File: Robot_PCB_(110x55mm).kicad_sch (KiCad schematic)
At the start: 24 parts, among them J1 HC-SR04, Q1 J3, SW1 Switch, U1 L293, U2 AMS1117-5.0, U5 MFRC522 37.5x25mm

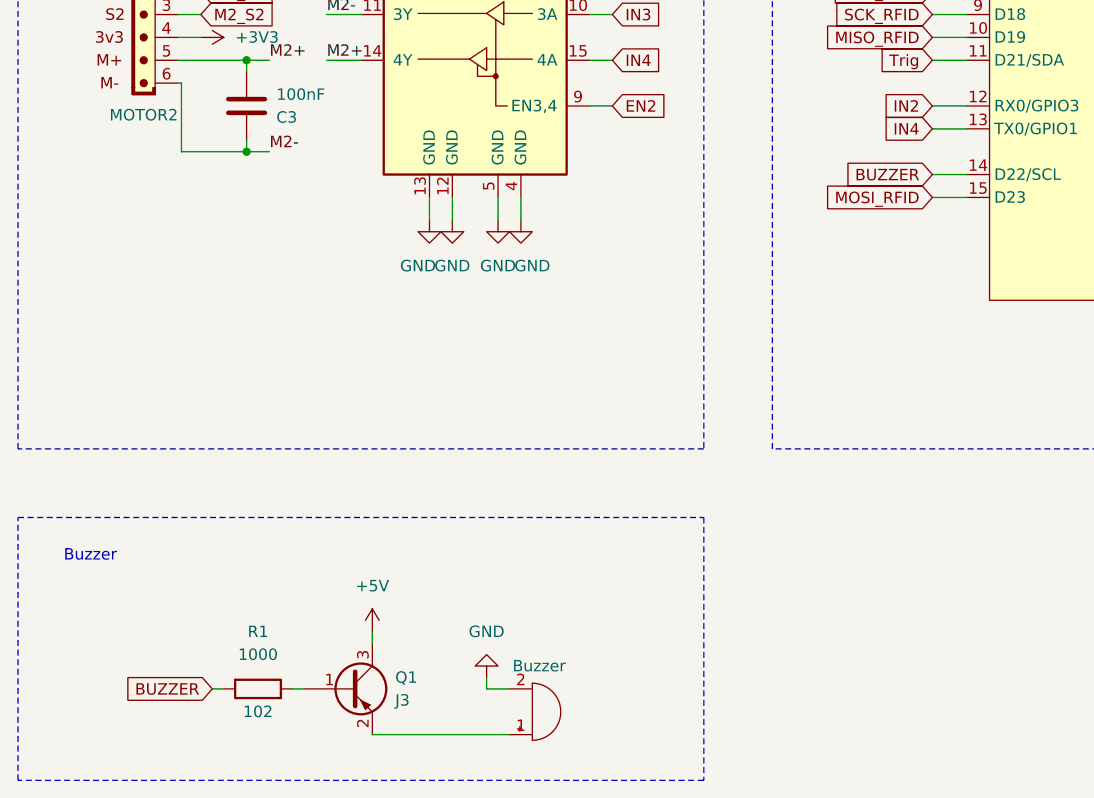
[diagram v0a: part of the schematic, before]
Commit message: Update
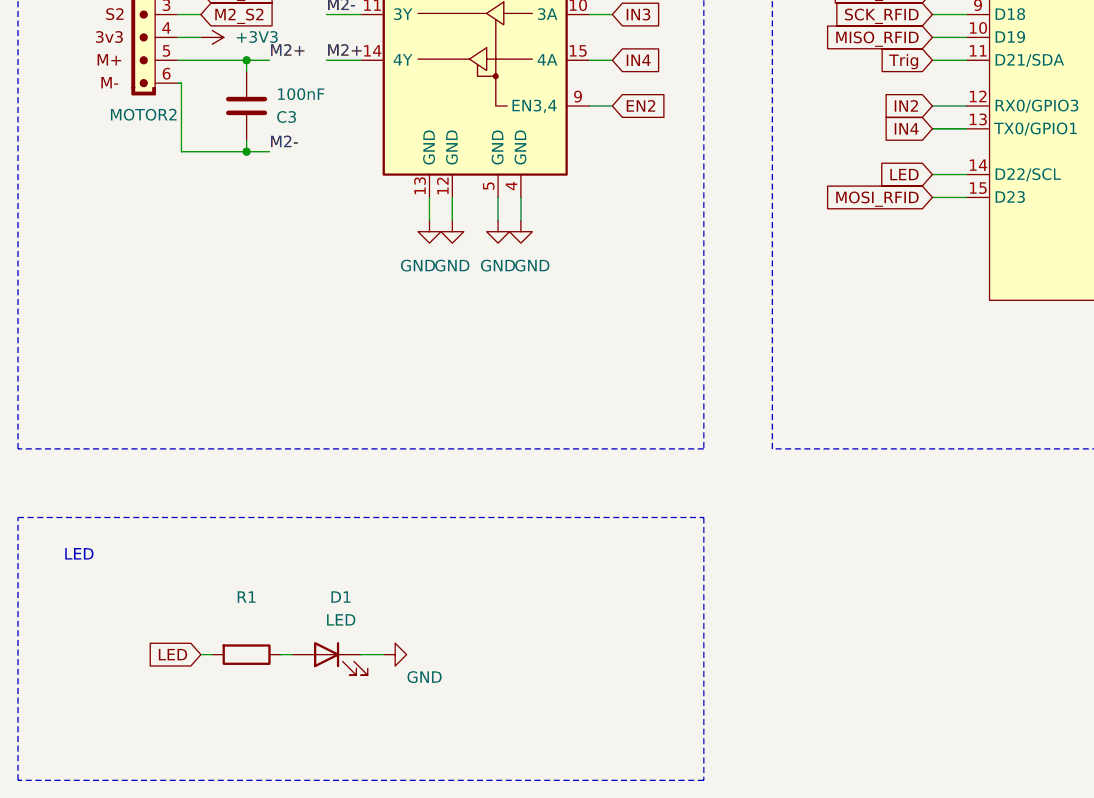
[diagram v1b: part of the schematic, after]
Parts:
- removed BZ1: Buzzer, Buzzer_Beeper:Buzzer_12x9.5RM7.6, symbol Device:Buzzer
- removed Q1: J3, Package_TO_SOT_SMD:SOT-23_Handsoldering, symbol Transistor_BJT:MMBT3906
- added D1: LED, LED_THT:LED_D3.0mm_Clear, symbol Device:LED
- R1: value 1000 -> ~; Campo4 102 -> (none)
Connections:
- net GND: now also D1.1 (K)
- net at R1.1: now also D1.2 (A)
- net BUZZER renamed LED
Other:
- note added: "LED"
- note removed: "Buzzer"
- moved on the sheet: R1
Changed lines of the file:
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@@
-    (stroke (width 0) (type default))
-  )
-  (wire (pts (xy 64.77 172.72) (xy 64.77 173.99))
-    (stroke (width 0) (type default))
-  )
-  (wire (pts (xy 64.77 184.15) (xy 80.01 184.15))
     (stroke (width 0) (type default))
   )
@@
     (stroke (width 0) (type default))
   )
-  (wire (pts (xy 77.47 177.8) (xy 77.47 179.07))
-    (stroke (width 0) (type default))
-  )
   (wire (pts (xy 200.66 44.45) (xy 210.82 44.45))
     (stroke (width 0) (type default))
@@
     (stroke (width 0) (type default))
   )
+  (wire (pts (xy 63.5 175.26) (xy 66.04 175.26))
+    (stroke (width 0) (type default))
+  )
   (wire (pts (xy 127 93.98) (xy 130.81 93.98))
     (stroke (width 0) (type default))
   )
-  (wire (pts (xy 46.99 179.07) (xy 48.26 179.07))
+  (wire (pts (xy 45.72 175.26) (xy 46.99 175.26))
     (stroke (width 0) (type default))
   )
@@
     (stroke (width 0) (type default))
   )
-  (wire (pts (xy 55.88 179.07) (xy 57.15 179.07))
-    (stroke (width 0) (type default))
-  )
   (wire (pts (xy 208.28 33.02) (xy 210.82 33.02))
     (stroke (width 0) (type default))
@@
     (stroke (width 0) (type default))
   )
-  (wire (pts (xy 77.47 179.07) (xy 80.01 179.07))
-    (stroke (width 0) (type default))
-  )
   (wire (pts (xy 91.44 93.98) (xy 88.9 93.98))
     (stroke (width 0) (type default))
@@
   )
   (wire (pts (xy 49.53 93.98) (xy 49.53 92.71))
+    (stroke (width 0) (type default))
+  )
+  (wire (pts (xy 55.88 175.26) (xy 54.61 175.26))
     (stroke (width 0) (type default))
   )
@@
     (effects (font (size 1.27 1.27)) (justify left bottom))
   )
-  (text "Buzzer" (at 30.48 165.1 0)
+  (text "LED" (at 30.48 165.1 0)
     (effects (font (size 1.27 1.27)) (justify left bottom))
   )
@@
     )
   )
-  (global_label "BUZZER" (shape input) (at 46.99 179.07 180) (fields_autoplaced)
-    (effects (font (size 1.27 1.27)) (justify right))
-    (property "Intersheetrefs" "${INTERSHEET_REFS}" (at 36.5663 179.07 0)
-      (effects (font (size 1.27 1.27)) (justify right) hide)
-    )
-  )
-  (global_label "BUZZER" (shape input) (at 127 121.92 180) (fields_autoplaced)
-    (effects (font (size 1.27 1.27)) (justify right))
-    (property "Intersheetrefs" "${INTERSHEET_REFS}" (at 116.5763 121.92 0)
+  (global_label "LED" (shape input) (at 45.72 175.26 180) (fields_autoplaced)
+    (effects (font (size 1.27 1.27)) (justify right))
+    (property "Intersheetrefs" "${INTERSHEET_REFS}" (at 39.2877 175.26 0)
+      (effects (font (size 1.27 1.27)) (justify right) hide)
+    )
+  )
+  (global_label "LED" (shape input) (at 127 121.92 180) (fields_autoplaced)
+    (effects (font (size 1.27 1.27)) (justify right))
+    (property "Intersheetrefs" "${INTERSHEET_REFS}" (at 120.5677 121.92 0)
       (effects (font (size 1.27 1.27)) (justify right) hide)
     )
@@
         (path "/5740c1d8-40a5-48a4-b0ff-1fed8540b5f6"
           (reference "#PWR030") (unit 1)
-        )
-      )
-    )
-  )
-  (symbol (lib_id "power:+5V") (at 64.77 172.72 0) (unit 1)
-    (in_bom yes) (on_board yes) (dnp no) (fields_autoplaced)
-    (property "Reference" "#PWR031" (at 64.77 176.53 0)
-      (effects (font (size 1.27 1.27)) hide)
-    )
-    (property "Value" "+5V" (at 64.77 167.64 0)
-      (effects (font (size 1.27 1.27)))
-    )
-    (property "Footprint" "" (at 64.77 172.72 0)
-      (effects (font (size 1.27 1.27)) hide)
-    )
-    (property "Datasheet" "" (at 64.77 172.72 0)
-      (effects (font (size 1.27 1.27)) hide)
-    )
-    (pin "1")
-    (instances
-      (project "Robot_PCB_(110x55mm)"
-        (path "/5740c1d8-40a5-48a4-b0ff-1fed8540b5f6"
-          (reference "#PWR031") (unit 1)
         )
       )
@@
     )
   )
+  (symbol (lib_id "power:GND") (at 66.04 175.26 90) (unit 1)
+    (in_bom yes) (on_board yes) (dnp no)
+    (property "Reference" "#PWR027" (at 72.39 175.26 0)
+      (effects (font (size 1.27 1.27)) hide)
+    )
+    (property "Value" "GND" (at 68.58 177.8 90)
+      (effects (font (size 1.27 1.27)) (justify right))
+    )
+    (property "Footprint" "" (at 66.04 175.26 0)
+      (effects (font (size 1.27 1.27)) hide)
+    )
+    (property "Datasheet" "" (at 66.04 175.26 0)
+      (effects (font (size 1.27 1.27)) hide)
+    )
+    (pin "1")
+    (instances
+      (project "Robot_PCB_(110x55mm)"
+        (path "/5740c1d8-40a5-48a4-b0ff-1fed8540b5f6"
+          (reference "#PWR027") (unit 1)
+        )
+      )
+    )
+  )
   (symbol (lib_id "Device:R") (at 247.65 34.29 0) (unit 1)
     (in_bom yes) (on_board yes) (dnp no)
@@
     )
   )
-  (symbol (lib_id "Device:R") (at 52.07 179.07 270) (unit 1)
-    (in_bom yes) (on_board yes) (dnp no)
-    (property "Reference" "R1" (at 52.07 172.72 90)
-      (effects (font (size 1.27 1.27)))
-    )
-    (property "Value" "1000" (at 52.07 175.26 90)
-      (effects (font (size 1.27 1.27)))
-    )
-    (property "Footprint" "Resistor_SMD:R_0805_2012Metric_Pad1.20x1.40mm_HandSolder" (at 52.07 177.292 90)
-      (effects (font (size 1.27 1.27)) hide)
-    )
-    (property "Datasheet" "~" (at 52.07 179.07 0)
-      (effects (font (size 1.27 1.27)) hide)
-    )
-    (property "Campo4" "102" (at 52.07 181.61 90)
-      (effects (font (size 1.27 1.27)))
+  (symbol (lib_id "Device:R") (at 50.8 175.26 270) (unit 1)
+    (in_bom yes) (on_board yes) (dnp no)
+    (property "Reference" "R1" (at 50.8 168.91 90)
+      (effects (font (size 1.27 1.27)))
+    )
+    (property "Value" "~" (at 50.8 171.45 90)
+      (effects (font (size 1.27 1.27)))
+    )
+    (property "Footprint" "Resistor_SMD:R_0805_2012Metric_Pad1.20x1.40mm_HandSolder" (at 50.8 173.482 90)
+      (effects (font (size 1.27 1.27)) hide)
+    )
+    (property "Datasheet" "~" (at 50.8 175.26 0)
+      (effects (font (size 1.27 1.27)) hide)
     )
     (pin "1")
@@
         (path "/5740c1d8-40a5-48a4-b0ff-1fed8540b5f6"
           (reference "#PWR04") (unit 1)
-        )
-      )
-    )
-  )
-  (symbol (lib_id "power:GND") (at 77.47 177.8 0) (mirror x) (unit 1)
-    (in_bom yes) (on_board yes) (dnp no)
-    (property "Reference" "#PWR027" (at 77.47 171.45 0)
-      (effects (font (size 1.27 1.27)) hide)
-    )
-    (property "Value" "GND" (at 77.47 172.72 0)
-      (effects (font (size 1.27 1.27)))
-    )
-    (property "Footprint" "" (at 77.47 177.8 0)
-      (effects (font (size 1.27 1.27)) hide)
-    )
-    (property "Datasheet" "" (at 77.47 177.8 0)
-      (effects (font (size 1.27 1.27)) hide)
-    )
-    (pin "1")
-    (instances
-      (project "Robot_PCB_(110x55mm)"
-        (path "/5740c1d8-40a5-48a4-b0ff-1fed8540b5f6"
-          (reference "#PWR027") (unit 1)
         )
       )
@@
     )
   )
-  (symbol (lib_id "Transistor_BJT:MMBT3906") (at 62.23 179.07 0) (unit 1)
-    (in_bom yes) (on_board yes) (dnp no) (fields_autoplaced)
-    (property "Reference" "Q1" (at 67.31 177.8 0)
-      (effects (font (size 1.27 1.27)) (justify left))
-    )
-    (property "Value" "J3" (at 67.31 180.34 0)
-      (effects (font (size 1.27 1.27)) (justify left))
-    )
-    (property "Footprint" "Package_TO_SOT_SMD:SOT-23_Handsoldering" (at 67.31 180.975 0)
-      (effects (font (size 1.27 1.27) italic) (justify left) hide)
-    )
-    (property "Datasheet" "https://www.onsemi.com/pdf/datasheet/pzt3906-d.pdf" (at 62.23 179.07 0)
-      (effects (font (size 1.27 1.27)) (justify left) hide)
-    )
-    (pin "1")
-    (pin "2")
-    (pin "3")
-    (instances
-      (project "Robot_PCB_(110x55mm)"
-        (path "/5740c1d8-40a5-48a4-b0ff-1fed8540b5f6"
-          (reference "Q1") (unit 1)
-        )
-      )
-    )
-  )
   (symbol (lib_id "power:GND") (at 259.08 76.2 90) (unit 1)
     (in_bom yes) (on_board yes) (dnp no)
@@
         (path "/5740c1d8-40a5-48a4-b0ff-1fed8540b5f6"
           (reference "#PWR029") (unit 1)
+        )
+      )
+    )
+  )
+  (symbol (lib_id "Device:LED") (at 59.69 175.26 0) (mirror y) (unit 1)
+    (in_bom yes) (on_board yes) (dnp no)
+    (property "Reference" "D1" (at 61.2775 168.91 0)
+      (effects (font (size 1.27 1.27)))
+    )
+    (property "Value" "LED" (at 61.2775 171.45 0)
+      (effects (font (size 1.27 1.27)))
+    )
+    (property "Footprint" "LED_THT:LED_D3.0mm_Clear" (at 59.69 175.26 0)
+      (effects (font (size 1.27 1.27)) hide)
+    )
+    (property "Datasheet" "~" (at 59.69 175.26 0)
+      (effects (font (size 1.27 1.27)) hide)
+    )
+    (pin "1")
+    (pin "2")
+    (instances
+      (project "Robot_PCB_(110x55mm)"
+        (path "/5740c1d8-40a5-48a4-b0ff-1fed8540b5f6"
+          (reference "D1") (unit 1)
         )
       )
@@
         )
       )
-    )
-  )
-  (symbol (lib_id "Device:Buzzer") (at 82.55 181.61 0) (mirror x) (unit 1)
-    (in_bom yes) (on_board yes) (dnp no)
-    (property "Reference" "BZ1" (at 82.0351 185.42 90)
-      (effects (font (size 1.27 1.27)) (justify left) hide)
-    )
-    (property "Value" "Buzzer" (at 83.3051 176.53 0)
-      (effects (font (size 1.27 1.27)))
-    )
-    (property "Footprint" "Buzzer_Beeper:Buzzer_12x9.5RM7.6" (at 81.915 184.15 90)
-      (effects (font (size 1.27 1.27)) hide)
-    )
-    (property "Datasheet" "~" (at 81.915 184.15 90)
-      (effects (font (size 1.27 1.27)) hide)
-    )
-    (pin "1")
-    (pin "2")
-    (instances
-      (project "Robot_PCB_(110x55mm)"
-        (path "/5740c1d8-40a5-48a4-b0ff-1fed8540b5f6"
-          (reference "BZ1") (unit 1)
-        )
-      )
